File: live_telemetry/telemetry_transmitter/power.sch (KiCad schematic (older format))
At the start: 36 parts, among them J2 Battery In, J3 BUS_CONN, Q1 Q_NMOS_GSD, Q2 Q_NMOS_GSD, Q3 Q_PMOS_GSD, Q4 Q_PMOS_GSD, Q5 Q_NMOS_GSD, U3 TLV70233QDBVRQ1, U5 INA180, U6 AP1509, U7 INA180

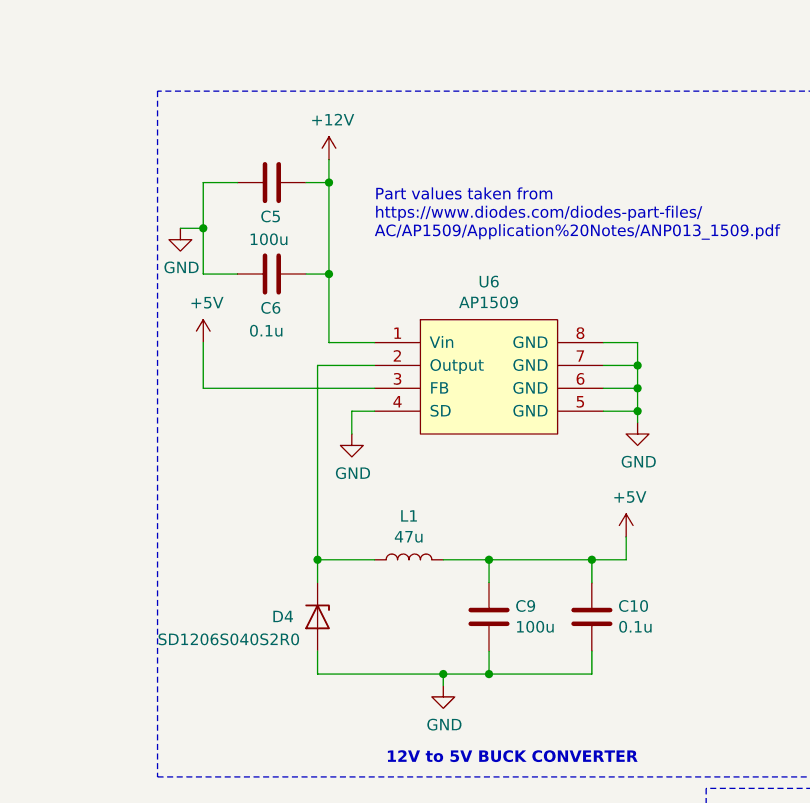
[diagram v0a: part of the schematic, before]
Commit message: Update LTT first pass layout
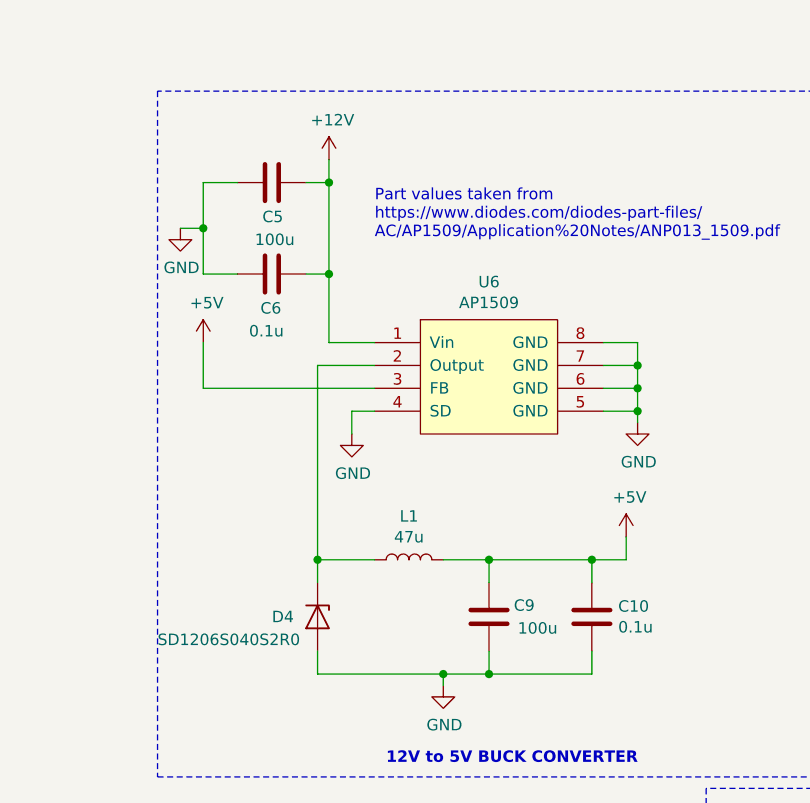
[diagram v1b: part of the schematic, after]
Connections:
- net +12V: now also C5.1; no longer C5.2
- net +5V: now also C9.1; no longer C9.2
- net GND: now also C5.2, C9.2; no longer C5.1, C9.1
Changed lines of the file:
@@
-$EndComp
-$Comp
-L Device:C C9
-U 1 1 5B9E08AC
-P 3000 3250
-F 0 "C9" H 2885 3204 50  0000 R CNN
-F 1 "100u" H 2885 3295 50  0000 R CNN
-F 2 "Capacitor_THT:CP_Radial_D7.5mm_P2.50mm" H 3038 3100 50  0001 C CNN
-F 3 "~" H 3000 3250 50  0001 C CNN
-	1    3000 3250
-	-1   0    0    1
 $EndComp
 $Comp
@@
 	2250 3000 2500 3000
 Wire Wire Line
-	3000 3100 3000 3000
-Wire Wire Line
 	3000 3000 2800 3000
 $Comp
@@
 U 1 1 5BB56714
 P 2050 1350
-F 0 "C5" V 1900 1400 50  0000 R CNN
-F 1 "100u" V 1800 1450 50  0000 R CNN
+F 0 "C5" V 2200 1400 50  0000 R CNN
+F 1 "100u" V 2300 1450 50  0000 R CNN
 F 2 "Capacitor_THT:CP_Radial_D7.5mm_P2.50mm" H 2088 1200 50  0001 C CNN
 F 3 "~" H 2050 1350 50  0001 C CNN
 	1    2050 1350
-	0    -1   -1   0
+	0    1    1    0
 $EndComp
 Wire Wire Line
@@
 Wire Wire Line
 	2800 3500 3000 3500
-Wire Wire Line
-	3000 3500 3000 3400
 Connection ~ 2800 3500
 Wire Wire Line
@@
 Wire Wire Line
 	8800 2650 9100 2650
+Wire Wire Line
+	3000 3100 3000 3000
+Wire Wire Line
+	3000 3500 3000 3400
+$Comp
+L Device:C C9
+U 1 1 5B9E08AC
+P 3000 3250
+F 0 "C9" H 3200 3300 50  0000 R CNN
+F 1 "100u" H 3300 3200 50  0000 R CNN
+F 2 "Capacitor_THT:CP_Radial_D7.5mm_P2.50mm" H 3038 3100 50  0001 C CNN
+F 3 "~" H 3000 3250 50  0001 C CNN
+	1    3000 3250
+	1    0    0    -1
+$EndComp
 $EndSCHEMATC
